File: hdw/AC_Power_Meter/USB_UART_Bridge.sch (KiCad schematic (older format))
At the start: 34 parts, among them J1001 USB_B_Mini, U1001 LT6700-1-S6, U1002 FT234XD, U1003 74LVC1G06, U1004 TPD3S014DBVR

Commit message: Updated most footprints
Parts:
- C1001, C1004, C1005, C1006, C1007, C1009, C1012, C1013, C1014: footprint (none) -> Capacitors_SMD:C_0603; Digi-Key PN PN -> 490-8020-1-ND
- C1002: footprint (none) -> Capacitors_SMD:C_0603; Digi-Key PN PN -> 1276-1921-1-ND
- C1003: footprint (none) -> Capacitors_SMD:C_0603; Digi-Key PN PN -> 478-1215-1-ND
- C1008: footprint (none) -> Capacitors_SMD:C_0805; Digi-Key PN PN -> 587-2990-1-ND; Voltage 10V -> 25V
- C1010, C1011: footprint (none) -> Capacitors_SMD:C_0603; Dielectric X7R -> C0G/NP0; Digi-Key PN PN -> 478-1171-1-ND
- D1001: footprint (none) -> LEDs:LED_0603; Digi-Key PN PN -> 160-1446-1-ND
- D1002: footprint (none) -> LEDs:LED_0603; Digi-Key PN PN -> 160-1448-1-ND
- J1001: footprint (none) -> Connectors:USB_Mini-B; Digi-Key PN (none) -> 732-2109-1-ND
- R1001: footprint (none) -> Resistors_SMD:R_0603; Digi-Key PN PN -> 311-487KHRCT-ND
- R1002: footprint (none) -> Resistors_SMD:R_0603; Digi-Key PN PN -> 311-6.04KHRCT-ND
- R1003: footprint (none) -> Resistors_SMD:R_0603; Digi-Key PN PN -> YAG3608CT-ND
- R1004, R1005: footprint (none) -> Resistors_SMD:R_0603; Digi-Key PN PN -> RHM10KADCT-ND
- R1006, R1009: footprint (none) -> Resistors_SMD:R_0603; Digi-Key PN PN -> MCT0603-1.00K-CFCT-ND
- TP1001: footprint (none) -> Measurement_Points:Measurement_Point_Round-SMD-Pad_Small

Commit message: Routed much more of the board, design rule fixes
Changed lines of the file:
@@
 Connection ~ 8190 2060
-Wire Wire Line
-	7690 2460 7690 3180
-Wire Wire Line
-	7790 2460 7790 3280
 Wire Wire Line
 	8680 2060 8680 2140
@@
 	3490 2740 3490 2780
 Connection ~ 3390 2740
-Wire Wire Line
-	7690 3180 9200 3180
 $Comp
 L Device:Ferrite_Bead L1001
@@
 Wire Wire Line
 	8930 2980 8570 2980
-Wire Wire Line
-	7790 3280 9200 3280
 Wire Wire Line
 	8930 2980 9200 2980
@@
 Wire Wire Line
 	5500 3180 5860 3180
-Connection ~ 7690 3180
-Wire Wire Line
-	7790 3280 6620 3280
-Connection ~ 7790 3280
 Wire Wire Line
 	5860 3570 5860 3180
 Connection ~ 5860 3180
-Wire Wire Line
-	5860 3180 7690 3180
 Wire Wire Line
 	6620 3570 6620 3280
@@
 Wire Wire Line
 	9600 3630 9600 3580
+Wire Wire Line
+	5860 3180 7790 3180
+Wire Wire Line
+	7690 2460 7690 3280
+Connection ~ 7690 3280
+Wire Wire Line
+	7690 3280 6620 3280
+Wire Wire Line
+	7690 3280 9200 3280
+Wire Wire Line
+	7790 3180 7790 2460
+Connection ~ 7790 3180
+Wire Wire Line
+	7790 3180 9200 3180
 $EndSCHEMATC

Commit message: Serious BOM scrubbing to drive price down
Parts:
- removed C1001, C1007: 0.1uF, Capacitors_SMD:C_0603, symbol Custom_Library:C_Custom
- removed C1002: 10nF, Capacitors_SMD:C_0603, symbol Custom_Library:C_Custom
- removed C1003: 1nF, Capacitors_SMD:C_0603, symbol Custom_Library:C_Custom
- removed D1001: Green, LEDs:LED_0603, symbol Custom_Library:LED_ALT_Custom
- removed R1001: 487k, Resistors_SMD:R_0603, symbol Custom_Library:R_Custom
- removed R1002: 6.04k, Resistors_SMD:R_0603, symbol Custom_Library:R_Custom
- removed R1003: 40.2k, Resistors_SMD:R_0603, symbol Custom_Library:R_Custom
- removed R1005: 10k, Resistors_SMD:R_0603, symbol Custom_Library:R_Custom
- removed R1006: 1k, Resistors_SMD:R_0603, symbol Custom_Library:R_Custom
- removed U1001: LT6700-1-S6, TO_SOT_Packages_SMD:TSOT-23-6, symbol Custom_Library:LT6700-1-S6
- removed U1003: 74LVC1G06, TO_SOT_Packages_SMD:SOT-353_SC-70-5, symbol Custom_Library:74LVC1G06_Power
- C1008: Digi-Key PN 587-2990-1-ND -> 478-10056-1-ND
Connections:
- wire segments 76 -> 51

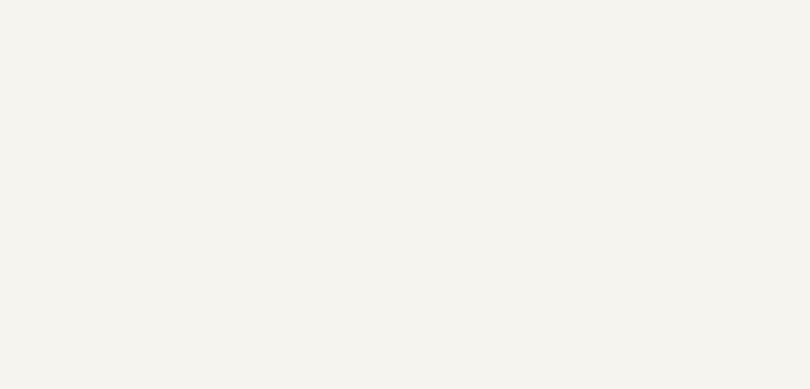
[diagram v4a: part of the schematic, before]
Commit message: Added a lot of functionality in formware
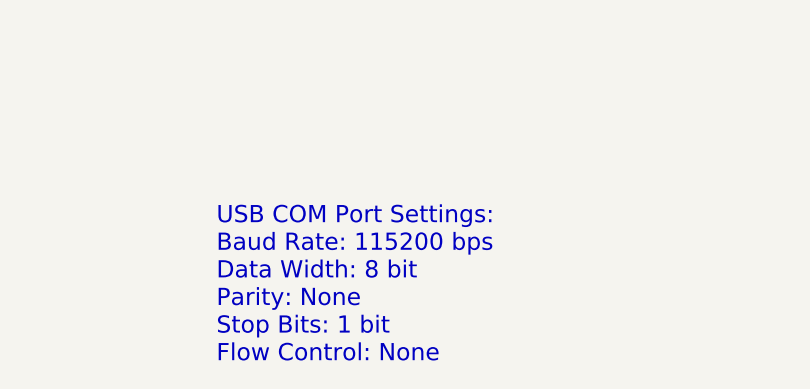
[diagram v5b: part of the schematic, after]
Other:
- note added: "USB COM Port Settings:\nBaud Rate: 115200 bps\nData Width: 8 bit\nParity: None\nStop Bits: 1 bit\nFlow Control: None"
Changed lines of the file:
@@
 Wire Wire Line
 	7790 3180 9200 3180
+Text Notes 2030 6200 0    75   ~ 0
+USB COM Port Settings:\nBaud Rate: 115200 bps\nData Width: 8 bit\nParity: None\nStop Bits: 1 bit\nFlow Control: None
 $EndSCHEMATC
